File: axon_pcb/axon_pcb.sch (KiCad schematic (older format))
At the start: 100 parts, among them J1 USB_C_Receptacle, J2 AVR_ISP Header, K1 KEYSW, K10 KEYSW, K11 KEYSW, K12 KEYSW, K13 KEYSW, K14 KEYSW, K15 KEYSW, K16 KEYSW, K17 KEYSW, K18 KEYSW, K19 KEYSW, K2 KEYSW, K20 KEYSW, K21 KEYSW, K22 KEYSW, K23 KEYSW, K24 KEYSW, K25 KEYSW, K26 KEYSW, K27 KEYSW, K28 KEYSW, K29 KEYSW, K3 KEYSW, K30 KEYSW, K31 KEYSW, K32 KEYSW, K33 KEYSW, K34 KEYSW, K35 KEYSW, K36 KEYSW, K37 KEYSW, K38 KEYSW, K39 KEYSW, K4 KEYSW, K40 KEYSW, K5 KEYSW, K6 KEYSW, K7 KEYSW, K8 KEYSW, K9 KEYSW, SW1 RESET, SW2 BOOT, U1 ATmega328P-PU, X1 16MHz

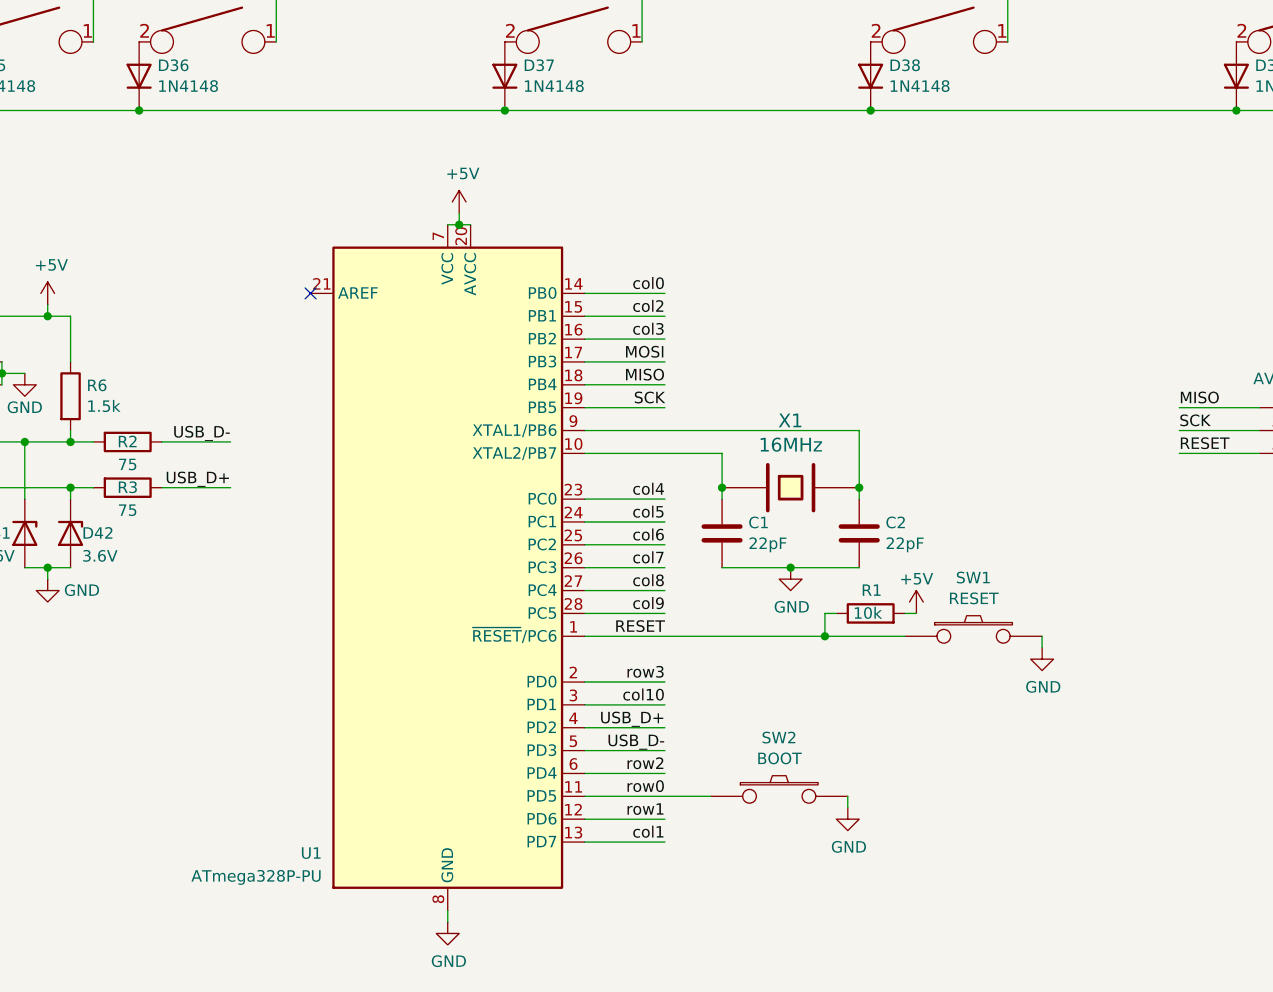
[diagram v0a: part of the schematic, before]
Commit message: fixed libraries, final pcb version
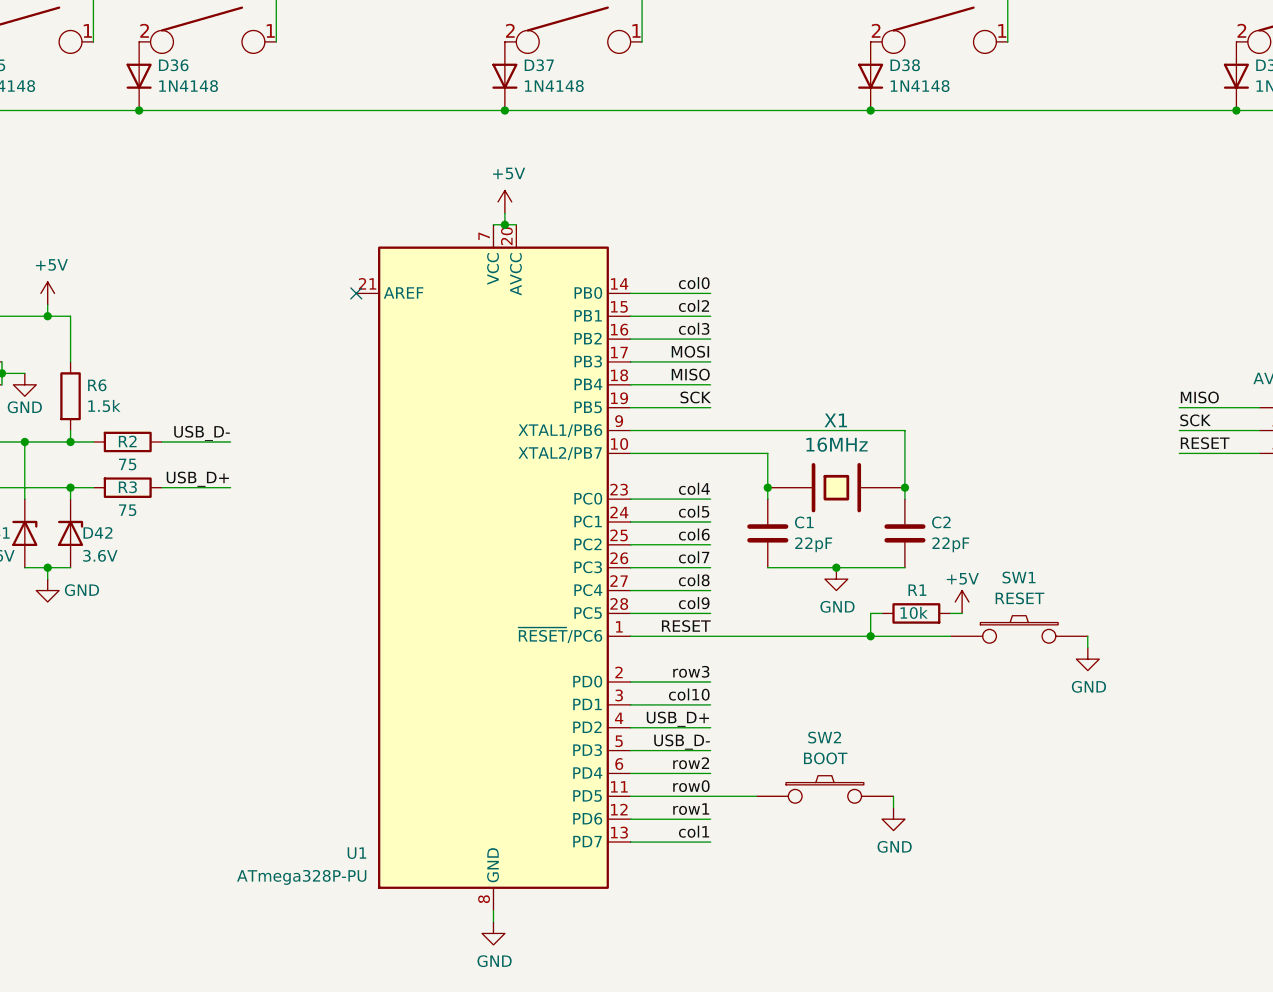
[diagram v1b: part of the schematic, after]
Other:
- moved on the sheet: C1, C2, R1, SW1, SW2, U1, X1
